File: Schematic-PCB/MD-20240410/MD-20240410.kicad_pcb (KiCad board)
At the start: 2 copper layers, 100.5 x 56.4 mm, 49 parts, among them J1 Conn_01x05_Pin, J2 Conn_01x04_Pin, J3 Conn_01x02_Pin, J4 Conn_01x02_Pin, J5 Conn_01x02_Pin, J6 Conn_01x02_Pin, J7 Conn_01x02_Pin, J8 Conn_01x15_Pin, Q3 NMOS, Q4 NMOS

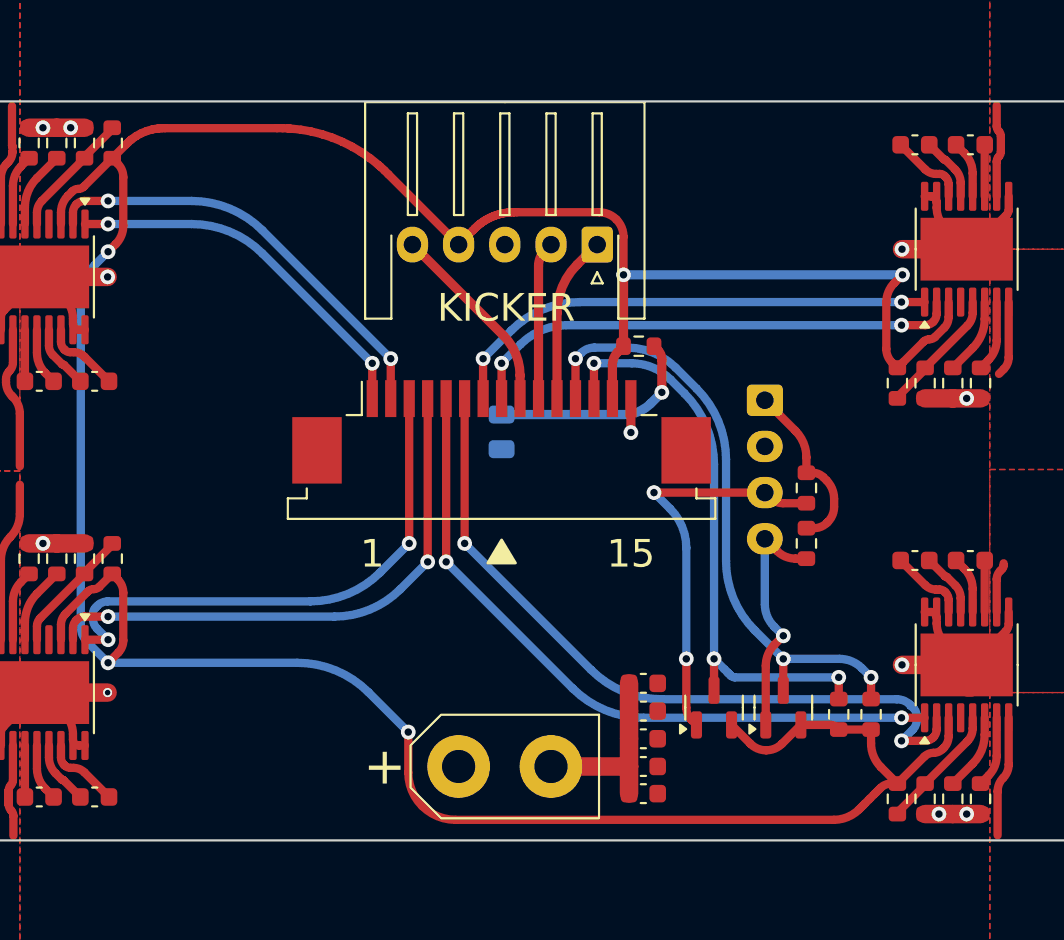
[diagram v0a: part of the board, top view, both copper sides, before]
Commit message: MDのDRしたよ
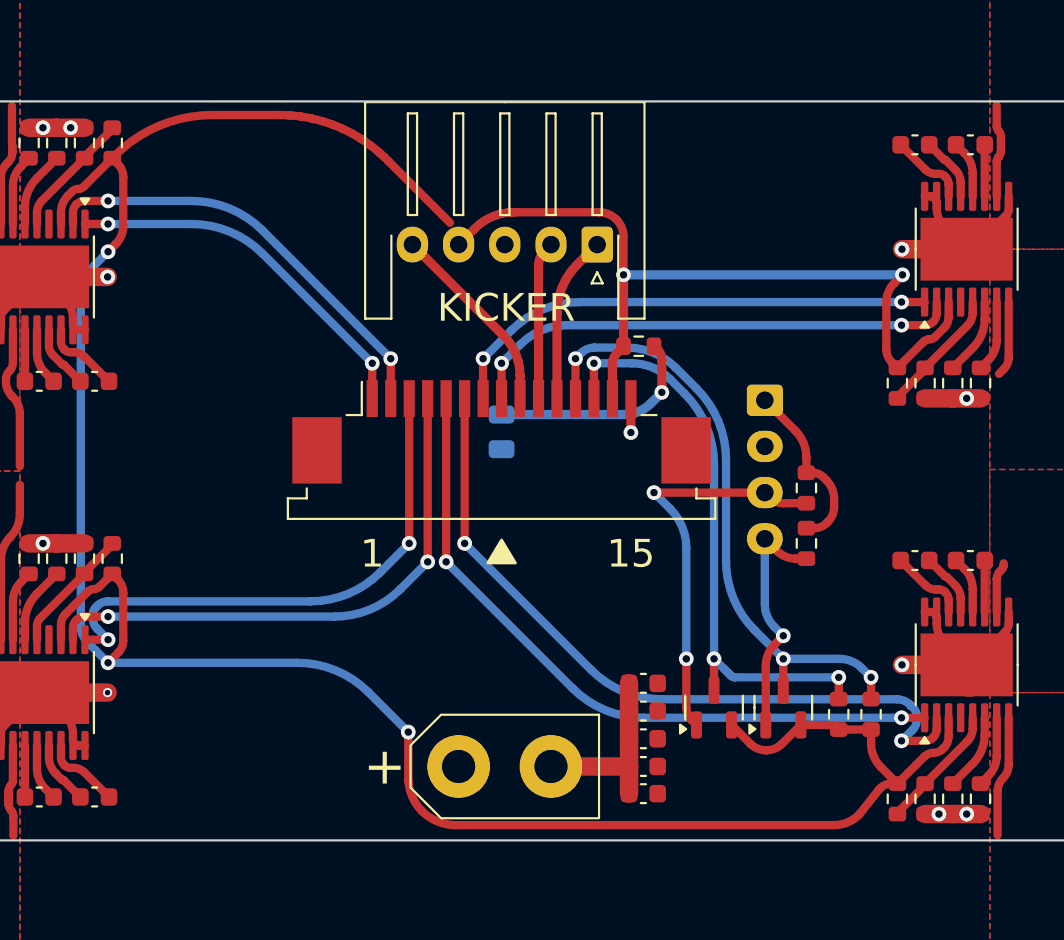
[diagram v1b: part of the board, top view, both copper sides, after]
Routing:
- net SLEEP-1: track 175.2 -> 175.8 mm

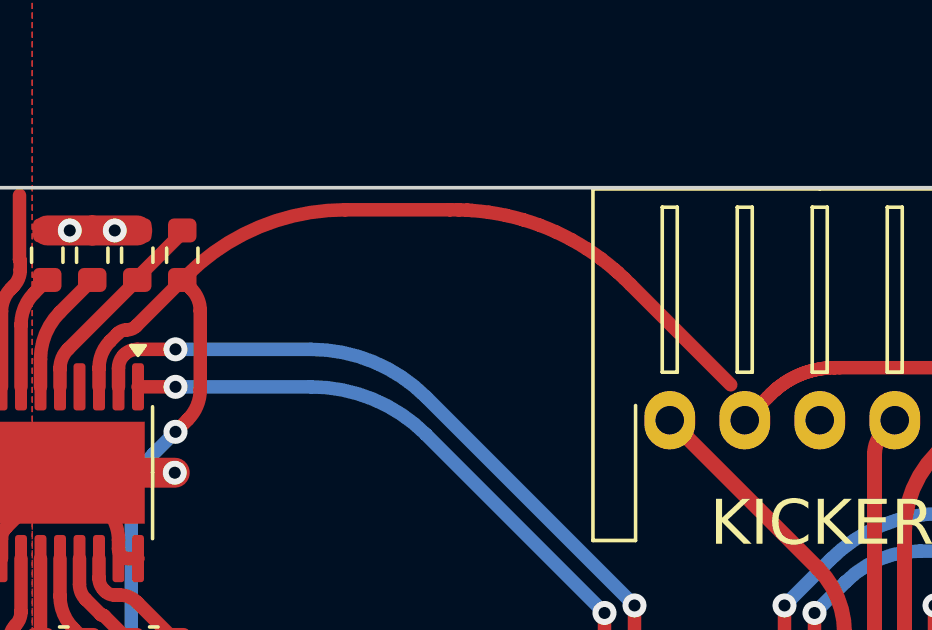
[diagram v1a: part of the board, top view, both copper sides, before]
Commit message: MD基板の再DRが完了した
製造用ファイル出力済み
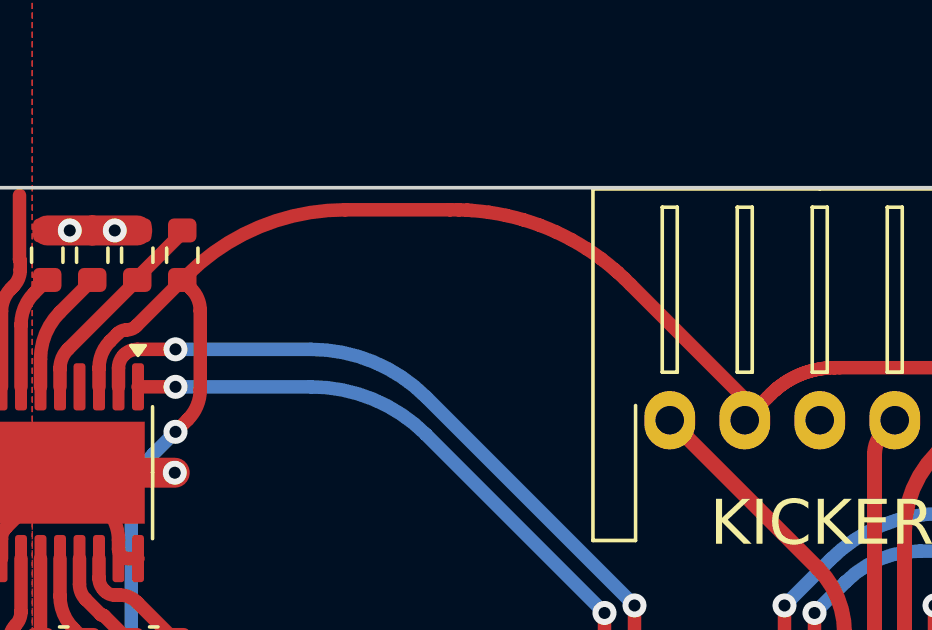
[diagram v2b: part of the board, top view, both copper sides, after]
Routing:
- net SLEEP-1: track 175.8 -> 177.8 mm
